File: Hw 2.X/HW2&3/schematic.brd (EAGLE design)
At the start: 160 x 100 mm, 23 parts, among them J1 USB-MB-H

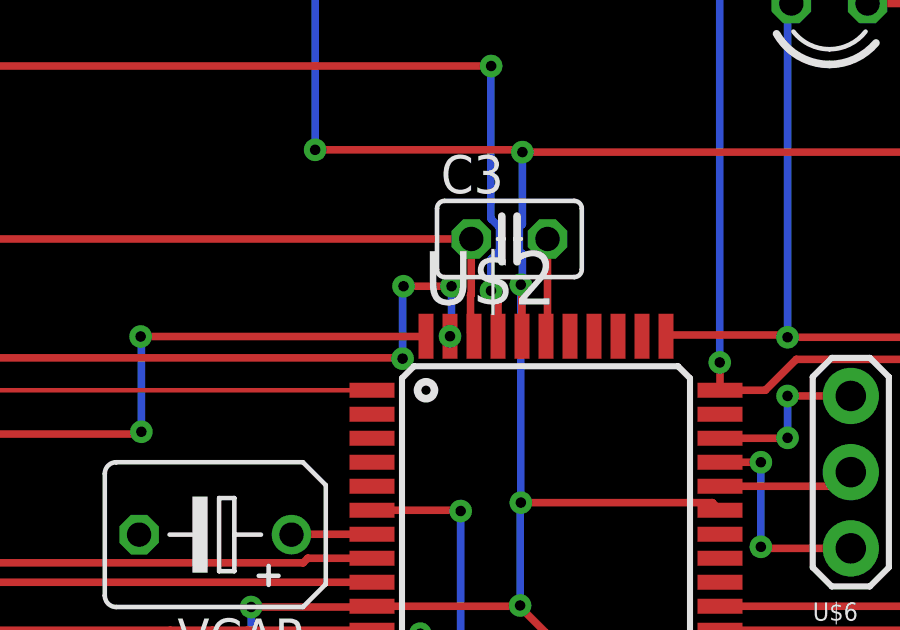
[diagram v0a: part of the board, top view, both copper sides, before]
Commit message: adjust board
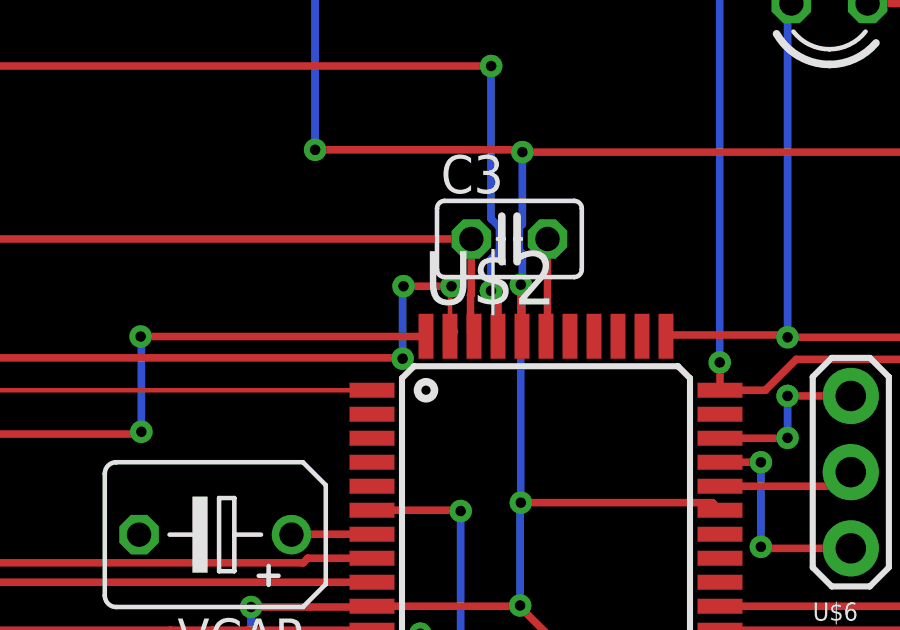
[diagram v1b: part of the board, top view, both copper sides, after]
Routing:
- net B7: track 74.7 -> 75.0 mm, vias 4 -> 3
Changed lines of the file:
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@@
 <wire x1="71.4502" y1="62.0776" x2="73.0504" y2="62.0776" width="0.254" layer="1"/>
 <via x="73.0504" y="62.0776" extent="1-16" drill="0.35"/>
-<wire x1="73.0504" y1="62.0776" x2="73.0504" y2="60.4604" width="0.254" layer="16"/>
-<wire x1="73.0504" y1="60.4604" x2="73" y2="60.41" width="0.254" layer="16"/>
-<via x="73" y="60.41" extent="1-16" drill="0.35"/>
+<wire x1="73.0504" y1="62.0776" x2="73.152" y2="61.976" width="0.254" layer="16"/>
+<wire x1="73.152" y1="60.562" x2="73" y2="60.41" width="0.254" layer="16"/>
+<wire x1="73.0504" y1="62.0776" x2="73" y2="62.0272" width="0.1524" layer="1"/>
+<wire x1="73" y1="62.0272" x2="73" y2="60.41" width="0.1524" layer="1"/>
+<wire x1="73" y1="60.41" x2="73" y2="60.41" width="0" layer="19" extent="1-16"/>
 </signal>
 <signal name="B8">
